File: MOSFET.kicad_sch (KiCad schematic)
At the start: 17 parts, among them Q1 CSD19532Q5B, Q2 CSD19532Q5B, Q3 CSD19532Q5B, Q4 CSD19532Q5B, Q5 CSD19532Q5B, Q7 CSD19532Q5B, U5 INA180B2

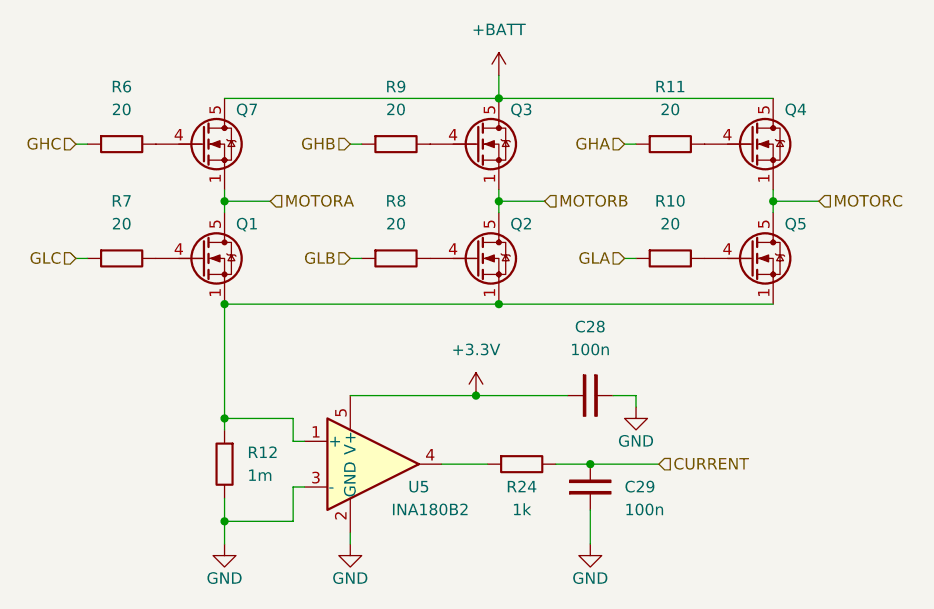
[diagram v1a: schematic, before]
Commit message: Add connectors,..
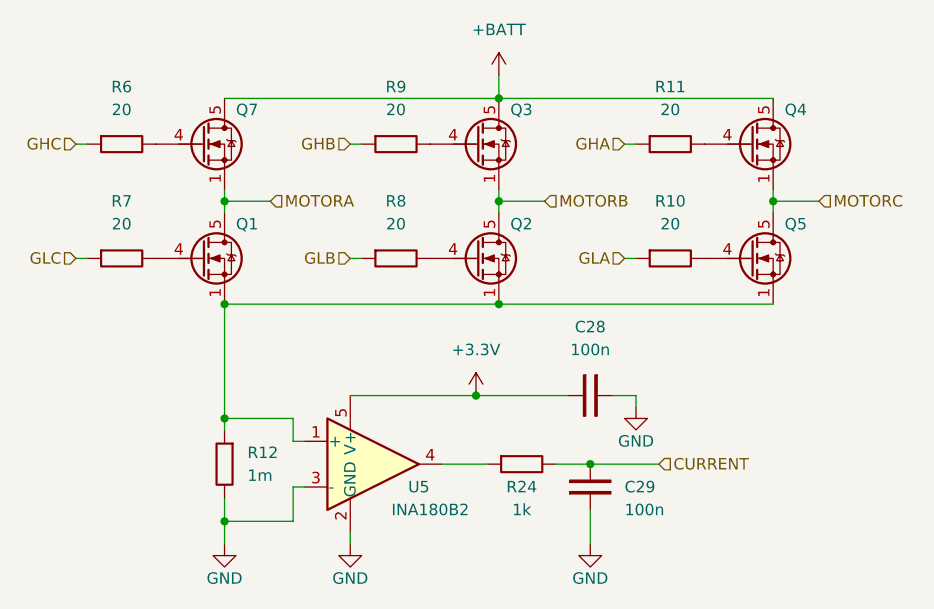
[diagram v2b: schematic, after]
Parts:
- C28, C29: footprint Capacitor_THT:C_Disc_D3.0mm_W2.0mm_P2.50mm -> Capacitor_SMD:C_0603_1608Metric_Pad1.08x0.95mm_HandSolder
- Q1, Q2, Q3, Q4, Q5, Q7: footprint Package_TO_SOT_SMD:TDSON-8-1 -> CSD19532Q5B:TRANS_CSD19532Q5B
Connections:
- net +3.3V: now also C28.2; no longer C28.1
- net GND: now also C28.1; no longer C28.2
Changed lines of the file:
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@@
 			)
 		)
-		(property "Footprint" "Package_TO_SOT_SMD:TDSON-8-1"
+		(property "Footprint" "CSD19532Q5B:TRANS_CSD19532Q5B"
 			(at 142.24 89.535 0)
 			(hide yes)
@@
 			)
 		)
-		(property "Footprint" "Package_TO_SOT_SMD:TDSON-8-1"
+		(property "Footprint" "CSD19532Q5B:TRANS_CSD19532Q5B"
 			(at 81.28 102.235 0)
 			(hide yes)
@@
 			)
 		)
-		(property "Footprint" "Package_TO_SOT_SMD:TDSON-8-1"
+		(property "Footprint" "CSD19532Q5B:TRANS_CSD19532Q5B"
 			(at 111.76 89.535 0)
 			(hide yes)
@@
 			)
 		)
-		(property "Footprint" "Capacitor_THT:C_Disc_D3.0mm_W2.0mm_P2.50mm"
+		(property "Footprint" "Capacitor_SMD:C_0603_1608Metric_Pad1.08x0.95mm_HandSolder"
 			(at 123.19 125.73 0)
 			(hide yes)
@@
 			)
 		)
-		(property "Footprint" "Package_TO_SOT_SMD:TDSON-8-1"
+		(property "Footprint" "CSD19532Q5B:TRANS_CSD19532Q5B"
 			(at 111.76 102.235 0)
 			(hide yes)
@@
 			)
 		)
-		(property "Footprint" "Package_TO_SOT_SMD:TDSON-8-1"
+		(property "Footprint" "CSD19532Q5B:TRANS_CSD19532Q5B"
 			(at 81.28 89.535 0)
 			(hide yes)
@@
 		(lib_id "PCM_SL_Devices:Capacitor_NP")
 		(at 119.38 115.57 0)
-		(unit 1)
-		(body_style 1)
-		(exclude_from_sim no)
-		(in_bom yes)
-		(on_board yes)
-		(in_pos_files yes)
-		(dnp no)
-		(fields_autoplaced yes)
+		(mirror y)
+		(unit 1)
+		(body_style 1)
+		(exclude_from_sim no)
+		(in_bom yes)
+		(on_board yes)
+		(in_pos_files yes)
+		(dnp no)
 		(property "Reference" "C28"
 			(at 119.38 107.95 0)
@@
 			)
 		)
-		(property "Footprint" "Capacitor_THT:C_Disc_D3.0mm_W2.0mm_P2.50mm"
+		(property "Footprint" "Capacitor_SMD:C_0603_1608Metric_Pad1.08x0.95mm_HandSolder"
 			(at 119.38 119.38 0)
 			(hide yes)
@@
 			)
 		)
-		(property "Footprint" "Package_TO_SOT_SMD:TDSON-8-1"
+		(property "Footprint" "CSD19532Q5B:TRANS_CSD19532Q5B"
 			(at 142.24 102.235 0)
 			(hide yes)
